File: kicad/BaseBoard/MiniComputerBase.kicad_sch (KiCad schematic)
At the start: 31 parts, among them J1 VIN, J2 PWRALT, J3 RESET, SW1 POWER, SW2 RESET, U1 L78L33, U2 LM7805, U3 W65C02SxP, X1 XTAL, X2 XTAL_ALT

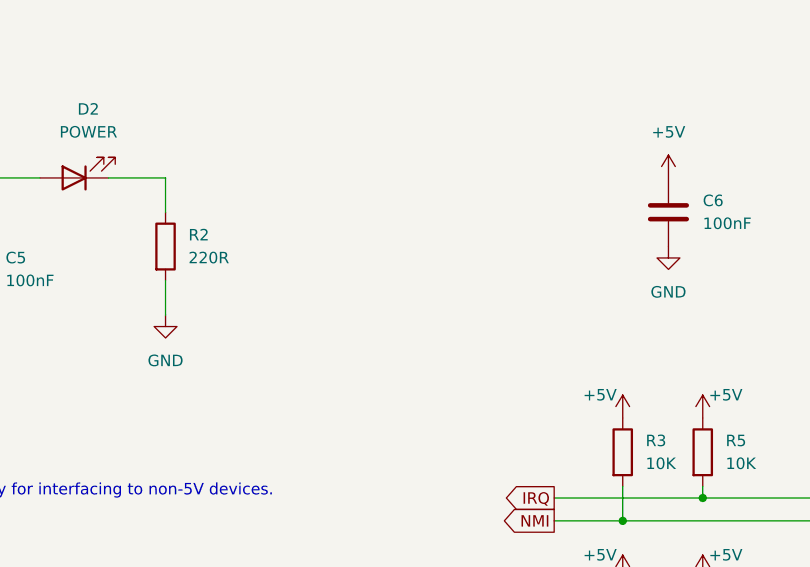
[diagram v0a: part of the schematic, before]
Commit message: Documentation
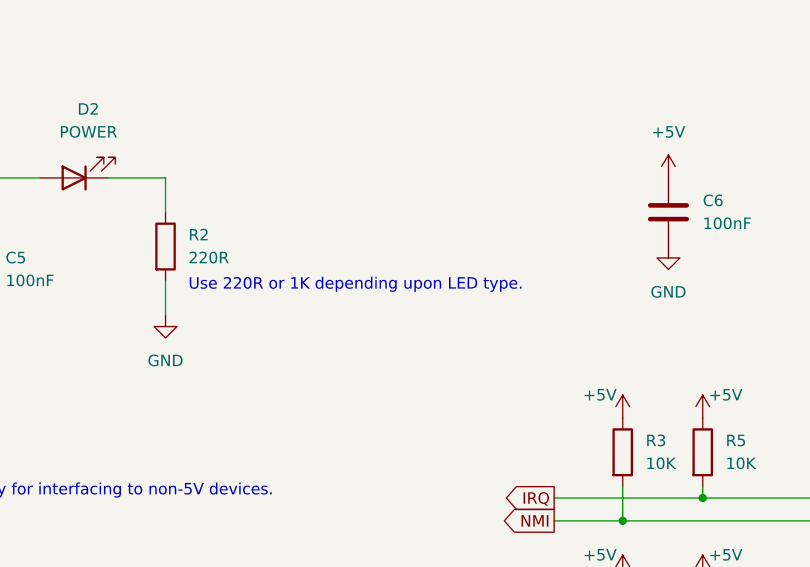
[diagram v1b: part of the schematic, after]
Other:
- note added: "Use 220R or 1K depending upon LED type."
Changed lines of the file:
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@@
+    (effects (font (size 1.27 1.27)) (justify left bottom))
+  )
+  (text "Use 220R or 1K depending upon LED type." (at 125.73 62.23 0)
     (effects (font (size 1.27 1.27)) (justify left bottom))
   )

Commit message: Component updates after first build
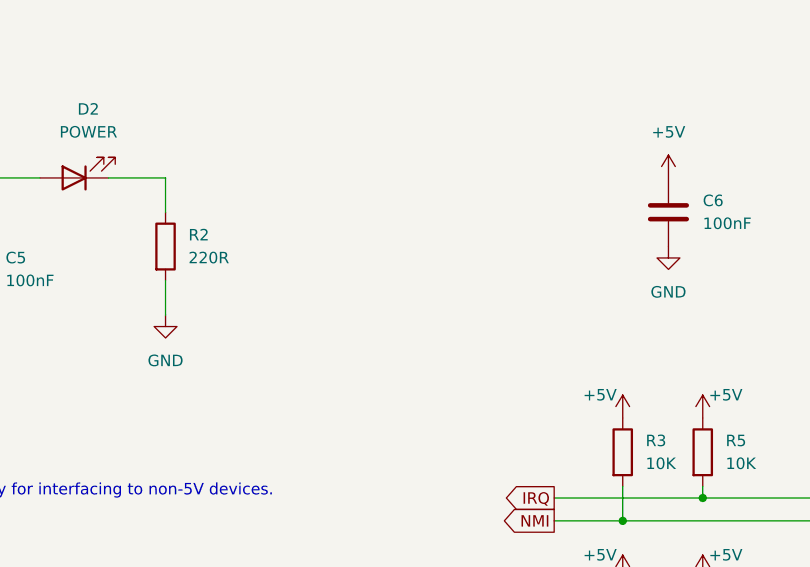
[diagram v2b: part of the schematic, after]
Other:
- note removed: "Use 220R or 1K depending upon LED type."
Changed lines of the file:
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@@
-    (effects (font (size 1.27 1.27)) (justify left bottom))
-  )
-  (text "Use 220R or 1K depending upon LED type." (at 125.73 62.23 0)
     (effects (font (size 1.27 1.27)) (justify left bottom))
   )
